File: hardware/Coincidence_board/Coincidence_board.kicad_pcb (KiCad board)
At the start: 2 copper layers, 136.8 x 92.5 mm, 69 parts, among them J1 Inputs, J3 POWER_IN, J4 Morpho_Gauche, J7 Morpho_Droite, SW1 SW_1, U1 74HCT74, U2 74HCT74, U3 LM7805_TO220, U4 74HC74, U5 74HC74, U6 74HC74, U7 74HC74

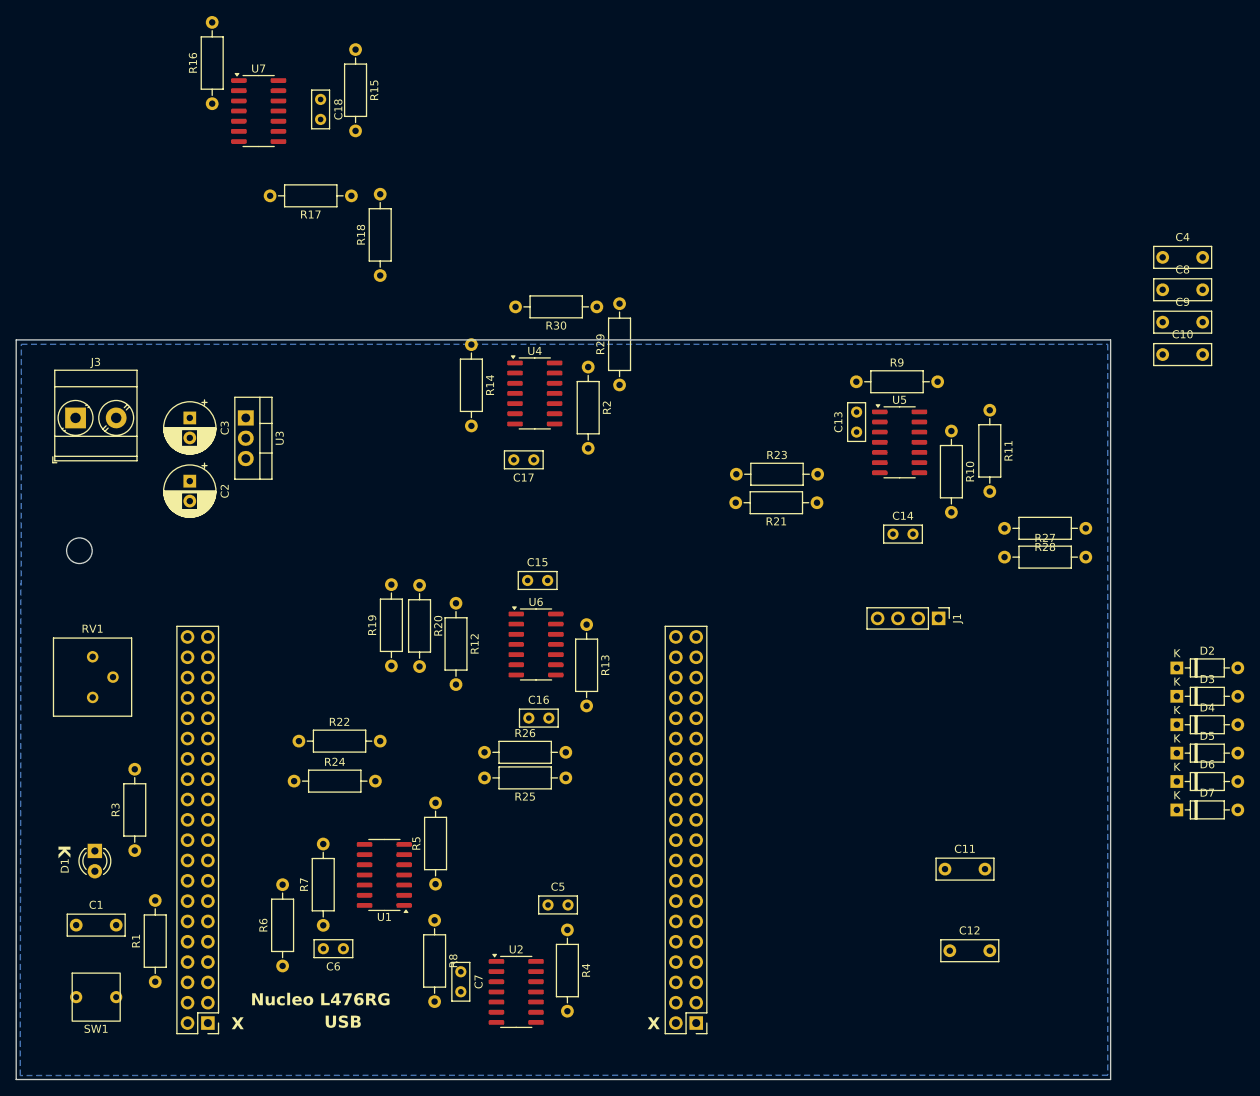
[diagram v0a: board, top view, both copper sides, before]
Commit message: Update Coincidence Board / Dephi 2024
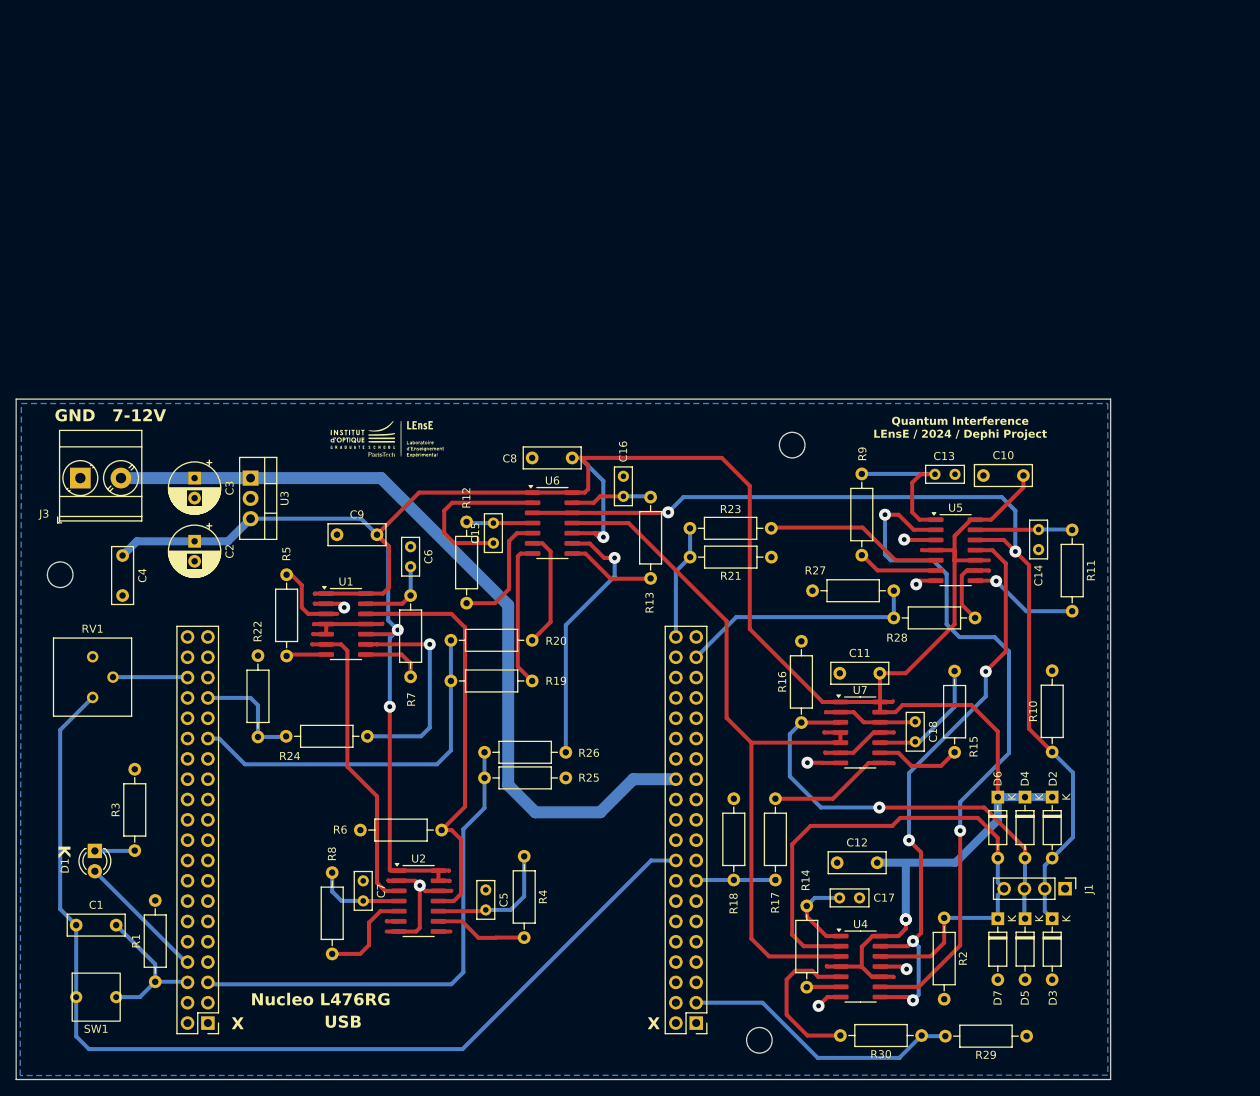
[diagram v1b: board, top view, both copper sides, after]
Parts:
- added ?: , , F.Cu at (220.5, 71.2)
- added ?: , , F.Cu at (216.4, 145.6)
- added G***: LOGO, LEnsE:Logo_Small, F.Cu at (169.9, 70.2)
- moved C4 135.2 mm to (136.8, 85.0), turned to -90 degrees
- moved U7 108.1 mm to (229.0, 107.1)
- moved R15 107.9 mm to (240.8, 99.4)
- moved C18 107.6 mm to (235.9, 105.8)
- moved R16 106.8 mm to (221.7, 105.9)
- moved C9 106.6 mm to (163.6, 82.4)
- moved R17 100.6 mm to (218.4, 125.6), turned to 90 degrees
- moved R30 99.7 mm to (236.7, 145.0)
- moved R29 96.0 mm to (249.8, 145.1), turned to 180 degrees
- moved U4 82.4 mm to (229.0, 136.4)
- moved R2 82.0 mm to (239.5, 130.3)
- moved R14 81.7 mm to (222.3, 128.8)
- moved R18 78.9 mm to (213.2, 115.4), turned to -90 degrees
- moved C8 76.7 mm to (193.0, 72.8), turned to 180 degrees
- moved C17 68.2 mm to (228.9, 127.8)
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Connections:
- J4 pad 15: unconnected-(J4-Pin_15-Pad15) -> B2out_nuc
- J4 pad 3: unconnected-(J4-Pin_3-Pad3) -> BC2out_nuc
- J4 pad 37: unconnected-(J4-Pin_37-Pad37) -> AC2out_nuc
- J4 pad 40: unconnected-(J4-Pin_40-Pad40) -> C2out_nuc
- J7 pad 13: ABCout_nuc -> unconnected-(J7-Pin_13-Pad13)
- J7 pad 26: AC2out_nuc -> unconnected-(J7-Pin_26-Pad26)
- J7 pad 29: unconnected-(J7-Pin_29-Pad29) -> A2out_nuc
- J7 pad 31: BC2out_nuc -> unconnected-(J7-Pin_31-Pad31)
- J7 pad 32: AB2out_nuc -> unconnected-(J7-Pin_32-Pad32)
- J7 pad 33: unconnected-(J7-Pin_33-Pad33) -> ABCout_nuc
- J7 pad 5: A2out_nuc -> AB2out_nuc
- J7 pad 7: B2out_nuc -> unconnected-(J7-Pin_7-Pad7)
- U1 pad 2: unconnected-(U1A-D-Pad2) -> GND
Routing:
- net 5V: track 0.00 -> 352.0 mm, vias 0 -> 5
- net 3.3V_NUC: track 0.00 -> 130.3 mm
- net A2in: track 0.00 -> 123.7 mm, vias 0 -> 2
- net VIN: track 0.00 -> 101.6 mm
- net GND: track 0.00 -> 95.4 mm, vias 0 -> 7
- net Net-(U4A-C): track 0.00 -> 91.9 mm
- net Net-(U4B-Q): track 0.00 -> 87.7 mm, vias 0 -> 2
- net C2in: track 0.00 -> 75.4 mm
- net Net-(U4B-~{Q}): track 0.00 -> 75.1 mm, vias 0 -> 4
- net AB2out_nuc: track 0.00 -> 61.3 mm
- net B2in: track 0.00 -> 54.2 mm, vias 0 -> 1
- net Ain: track 0.00 -> 52.5 mm
- net A2out_nuc: track 0.00 -> 46.2 mm
- net Net-(U1A-~{Q}): track 0.00 -> 38.4 mm
- net BC2out_nuc: track 0.00 -> 35.2 mm
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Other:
- board size 136.8 x 92.5 mm -> 136.8 x 85 mm
- board text added: "7-12V"
- board text added: "GND"
- board text added: "Quantum Interference LEnsE / 2024 / Dephi Project"
